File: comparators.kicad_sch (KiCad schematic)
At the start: 77 parts, among them SW7 SW_DIP_x03, U41 TLV3502AIDR, U42 TLV3502AIDR, U43 TLV3502AIDR, U44 TLV3502AIDR, U45 TLV3502AIDR, U46 TLV3502AIDR, U47 TLV3502AIDR, U48 TLV3502AIDR, U49 TLV3502AIDR, U50 TLV3502AIDR, U51 TLV3502AIDR, U52 TLV3502AIDR, U53 TXB0108PW, U54 TXB0108PW, U55 TXB0108PW

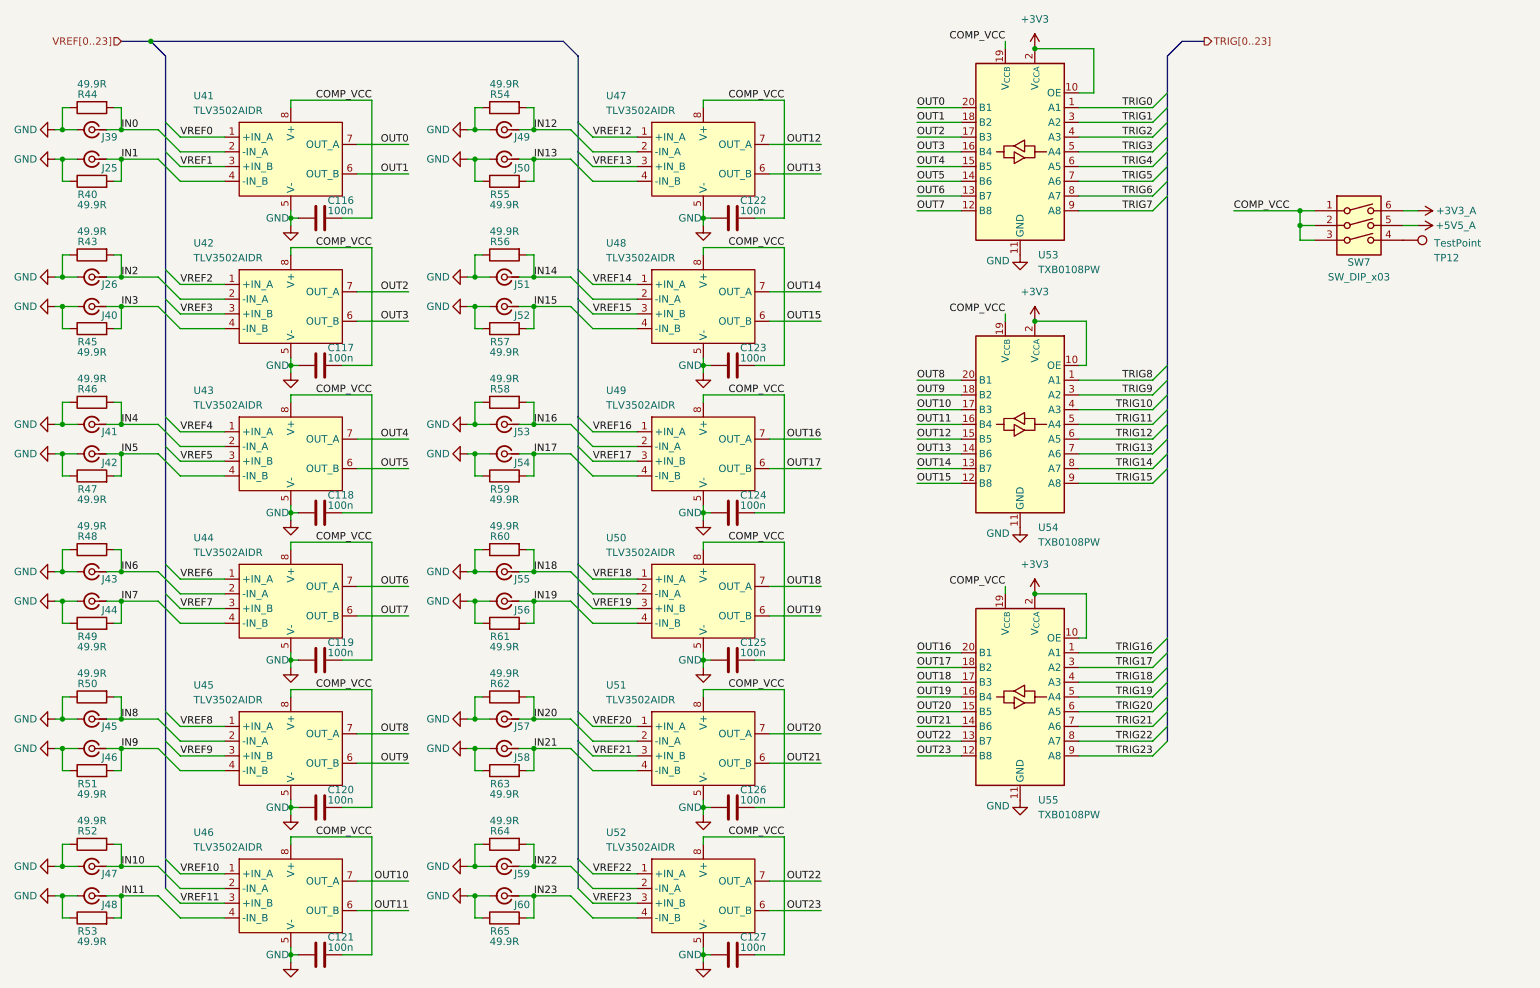
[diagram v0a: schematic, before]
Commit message: series resistors
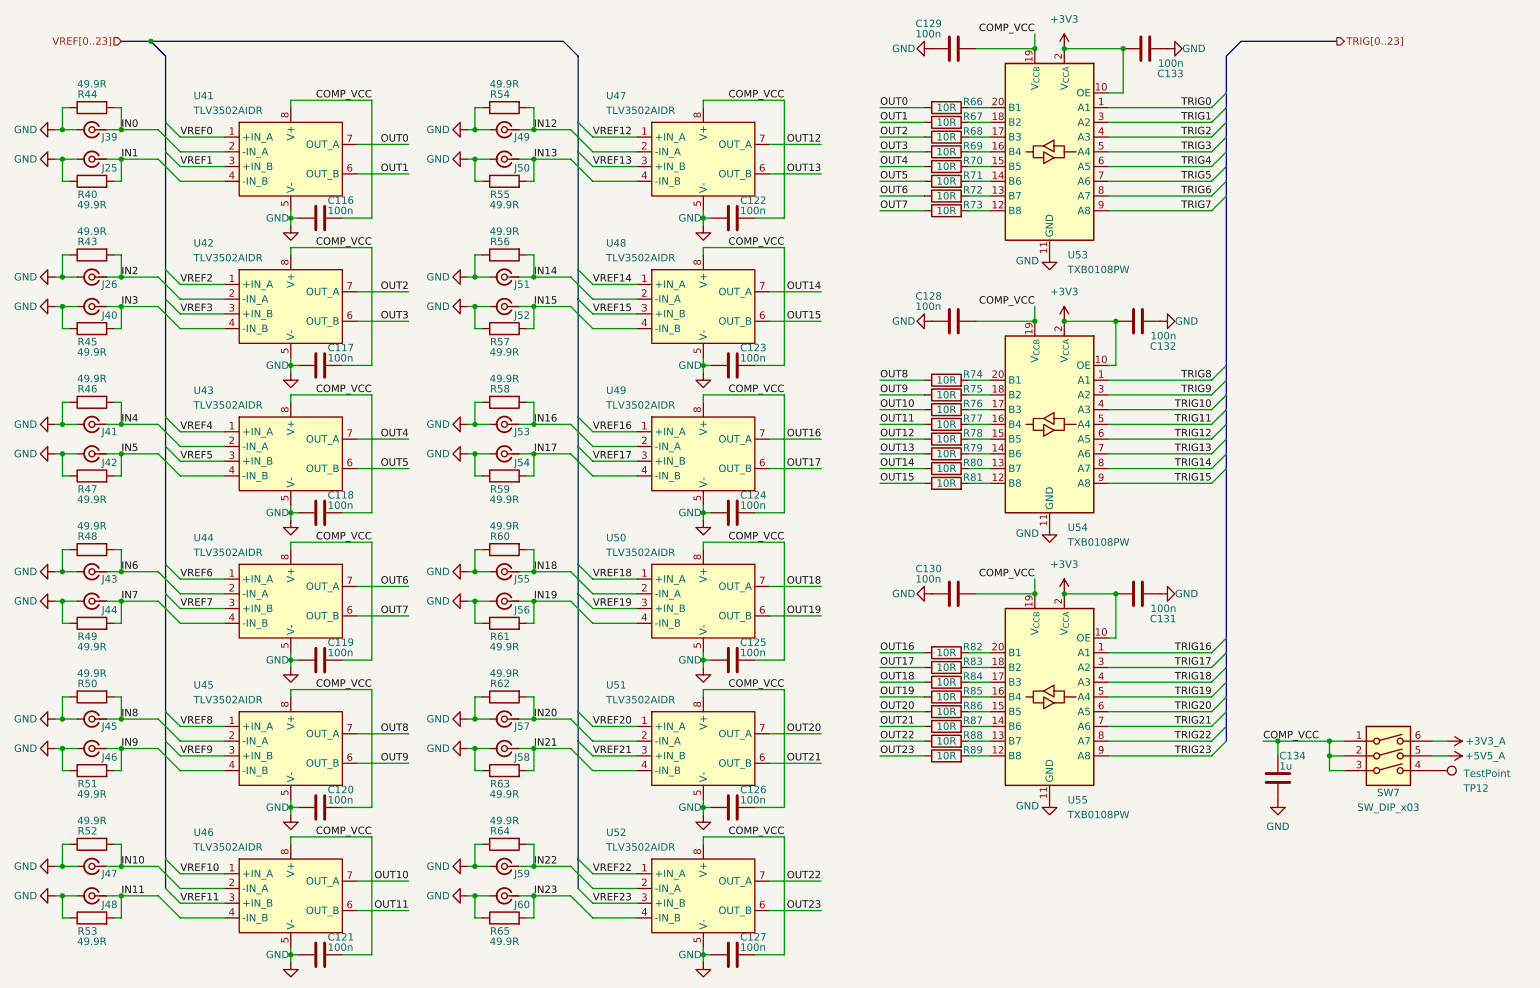
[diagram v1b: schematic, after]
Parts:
- added C128, C129, C130, C131, C132, C133: 100n, symbol Device:C
- added C134: 1u, symbol Device:C
- added R66, R67, R68, R69, R70, R71, R72, R73, R74, R75, R76, R77, R78, R79, R80, R81, R82, R83, R84, R85, R86, R87, R88, R89: 10R, symbol Device:R
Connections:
- net +3V3: now also C131.1, C132.1, C133.1
- net COMP_VCC: now also C128.1, C129.1, C130.1, C134.1
- net GND: now also C128.2, C129.2, C130.2, C131.2, C132.2, C133.2, C134.2
- net OUT0: now also R66.1; no longer U53.20 (B1)
- net OUT1: now also R67.1; no longer U53.18 (B2)
- net OUT10: now also R76.1; no longer U54.17 (B3)
- net OUT11: now also R77.1; no longer U54.16 (B4)
- net OUT12: now also R78.1; no longer U54.15 (B5)
- net OUT13: now also R79.1; no longer U54.14 (B6)
- net OUT14: now also R80.1; no longer U54.13 (B7)
- net OUT15: now also R81.1; no longer U54.12 (B8)
- net OUT16: now also R82.1; no longer U55.20 (B1)
- net OUT17: now also R83.1; no longer U55.18 (B2)
- net OUT18: now also R84.1; no longer U55.17 (B3)
- net OUT19: now also R85.1; no longer U55.16 (B4)
- net OUT2: now also R68.1; no longer U53.17 (B3)
- net OUT20: now also R86.1; no longer U55.15 (B5)
- net OUT21: now also R87.1; no longer U55.14 (B6)
- net OUT22: now also R88.1; no longer U55.13 (B7)
- net OUT23: now also R89.1; no longer U55.12 (B8)
- net OUT3: now also R69.1; no longer U53.16 (B4)
- net OUT4: now also R70.1; no longer U53.15 (B5)
- net OUT5: now also R71.1; no longer U53.14 (B6)
- net OUT6: now also R72.1; no longer U53.13 (B7)
- net OUT7: now also R73.1; no longer U53.12 (B8)
- net OUT8: now also R74.1; no longer U54.20 (B1)
- net OUT9: now also R75.1; no longer U54.18 (B2)
- new net: R67.2, U53.18 (B2)
- new net: R81.2, U54.12 (B8)
- new net: R80.2, U54.13 (B7)
- new net: R79.2, U54.14 (B6)
- new net: R78.2, U54.15 (B5)
- new net: R77.2, U54.16 (B4)
- new net: R76.2, U54.17 (B3)
- new net: R75.2, U54.18 (B2)
- new net: R74.2, U54.20 (B1)
- new net: R73.2, U53.12 (B8)
- new net: R72.2, U53.13 (B7)
- new net: R71.2, U53.14 (B6)
- new net: R70.2, U53.15 (B5)
- new net: R69.2, U53.16 (B4)
- new net: R68.2, U53.17 (B3)
- new net: R66.2, U53.20 (B1)
- new net: R85.2, U55.16 (B4)
- new net: R88.2, U55.13 (B7)
- new net: R83.2, U55.18 (B2)
- new net: R89.2, U55.12 (B8)
- new net: R87.2, U55.14 (B6)
- new net: R86.2, U55.15 (B5)
- new net: R84.2, U55.17 (B3)
- new net: R82.2, U55.20 (B1)
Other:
- moved on the sheet: SW7, TP12, U53, U54, U55
